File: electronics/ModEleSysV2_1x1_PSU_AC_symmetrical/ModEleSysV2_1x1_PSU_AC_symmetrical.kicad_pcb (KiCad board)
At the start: 2 copper layers, 43.2 x 49.5 mm, 30 parts, among them J2 Jack-DC, SW1 switch_DPDT, U1 LM317, U2 LM337

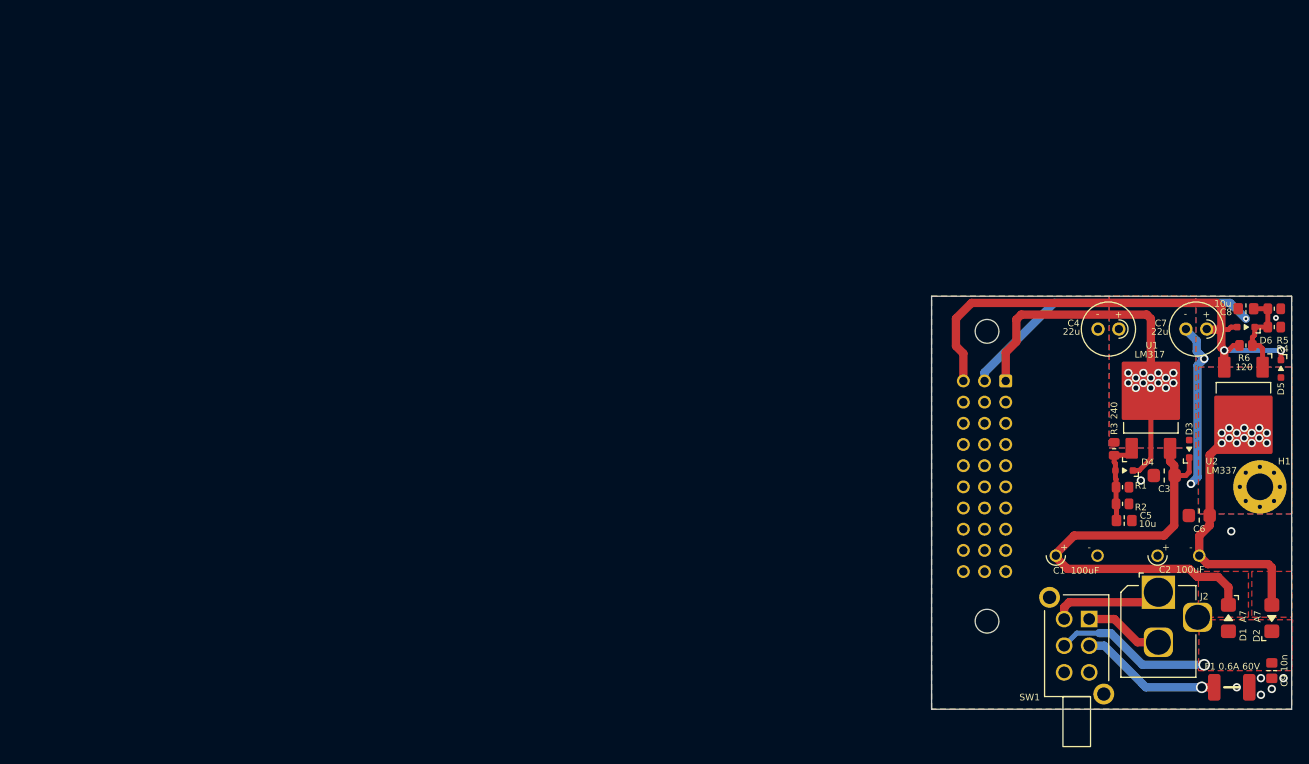
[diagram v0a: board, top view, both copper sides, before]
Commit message: reviewed and updated PCB's
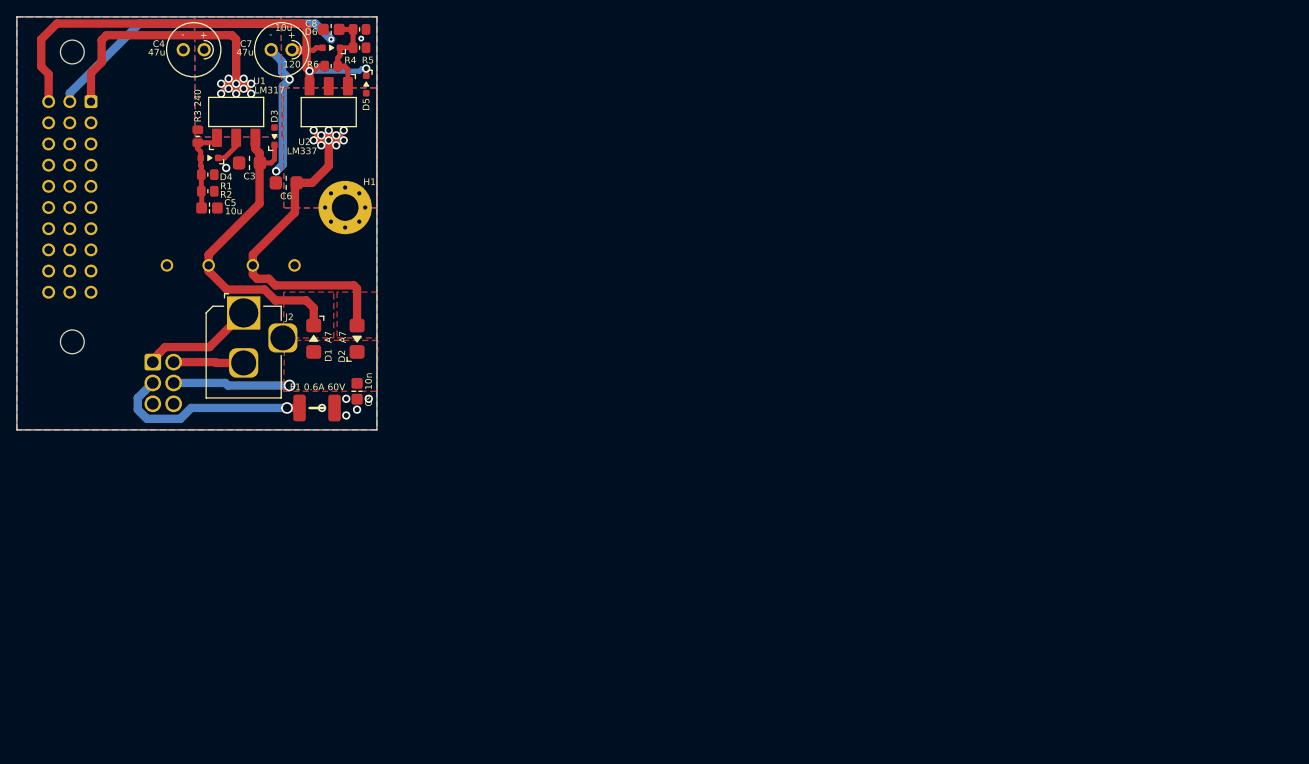
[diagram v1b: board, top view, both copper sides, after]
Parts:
- removed SW1: switch_DPDT, SquantorSwitches:PS-22F02
- added J3: PINS_2X03, SquantorConnectors:DLL-XHY-6A, B.Cu at (47.5, 73.9)
- C1, C2: moved to B.Cu
- C4, C7: value 22u -> 47u
- U1, U2: footprint SquantorIC:TO-252_D-PAK_IRF -> SquantorIC:SOT-223
- moved C6 116.5 mm to (62.3, 49.9)
- moved R3 116.1 mm to (51.7, 44.3)
- moved U2 115.9 mm to (67.4, 41.4)
- moved C5 115.9 mm to (53.1, 52.9)
- moved D4 115.9 mm to (53.1, 46.9)
- moved C3 115.9 mm to (57.9, 47.5)
- moved D3 115.9 mm to (60.9, 44.3)
- moved R1 115.9 mm to (52.9, 48.9)
- moved R2 115.9 mm to (52.9, 50.9)
- moved D5 114.9 mm to (71.9, 38.1)
- moved D1 114.7 mm to (65.6, 68.6)
- moved J1 114.7 mm to (36.4, 51.6)
- moved R4 114.7 mm to (71.1, 33.7)
- moved R5 114.7 mm to (71.1, 31.5)
- moved C8 114.7 mm to (67.7, 31.5)
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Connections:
- J2 pad 1: /AC_PHASE1_IN -> /AC_NEUT_IN
- J2 pad 2: /AC_NEUT_IN -> /AC_PHASE1_IN
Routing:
- net /DC1p: track 53.5 -> 39.2 mm
- net /DC1n: track 28.6 -> 38.6 mm, vias 14 -> 10
- net /+aV: track 42.5 -> 32.5 mm, vias 14 -> 10
- net Net-(F1-Pad1): track 17.1 -> 24.3 mm
- net /AC_PHASE1_IN: track 13.5 -> 8.44 mm
- net /AC1_PHASE: track 19.0 -> 14.0 mm
- net /AC_NEUT_IN: track 9.46 -> 13.5 mm
- net GND: track 56.7 -> 52.8 mm, vias 11 -> 10
